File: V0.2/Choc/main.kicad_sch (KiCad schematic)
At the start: 40 parts, among them J1 USB_C_2.0, J2 JST-BAT, J3 SWD, SW1 SW_DPST_x2, SW10 SW_DPST_x2, SW11 SW_DPST_x2, SW12 SW_DPST_x2, SW13 SW_DPST_x2, SW14 SW_DPST_x2, SW15 SW_DPST_x2, SW16 SW_DPST_x2, SW17 SW_DPST_x2, SW18 SW_DPST_x2, SW19 SW_DPST_x2, SW2 SW_DPST_x2, SW20 SW_DPST_x2, SW21 SW_DPST_x2, SW3 SW_DPST_x2, SW4 SW_DPST_x2, SW5 SW_DPST_x2, SW6 SW_DPST_x2, SW7 SW_DPST_x2, SW8 SW_DPST_x2, SW9 SW_DPST_x2, U1 IP4234CZ6, U2 BQ24072, U3 MS88SF31_Min

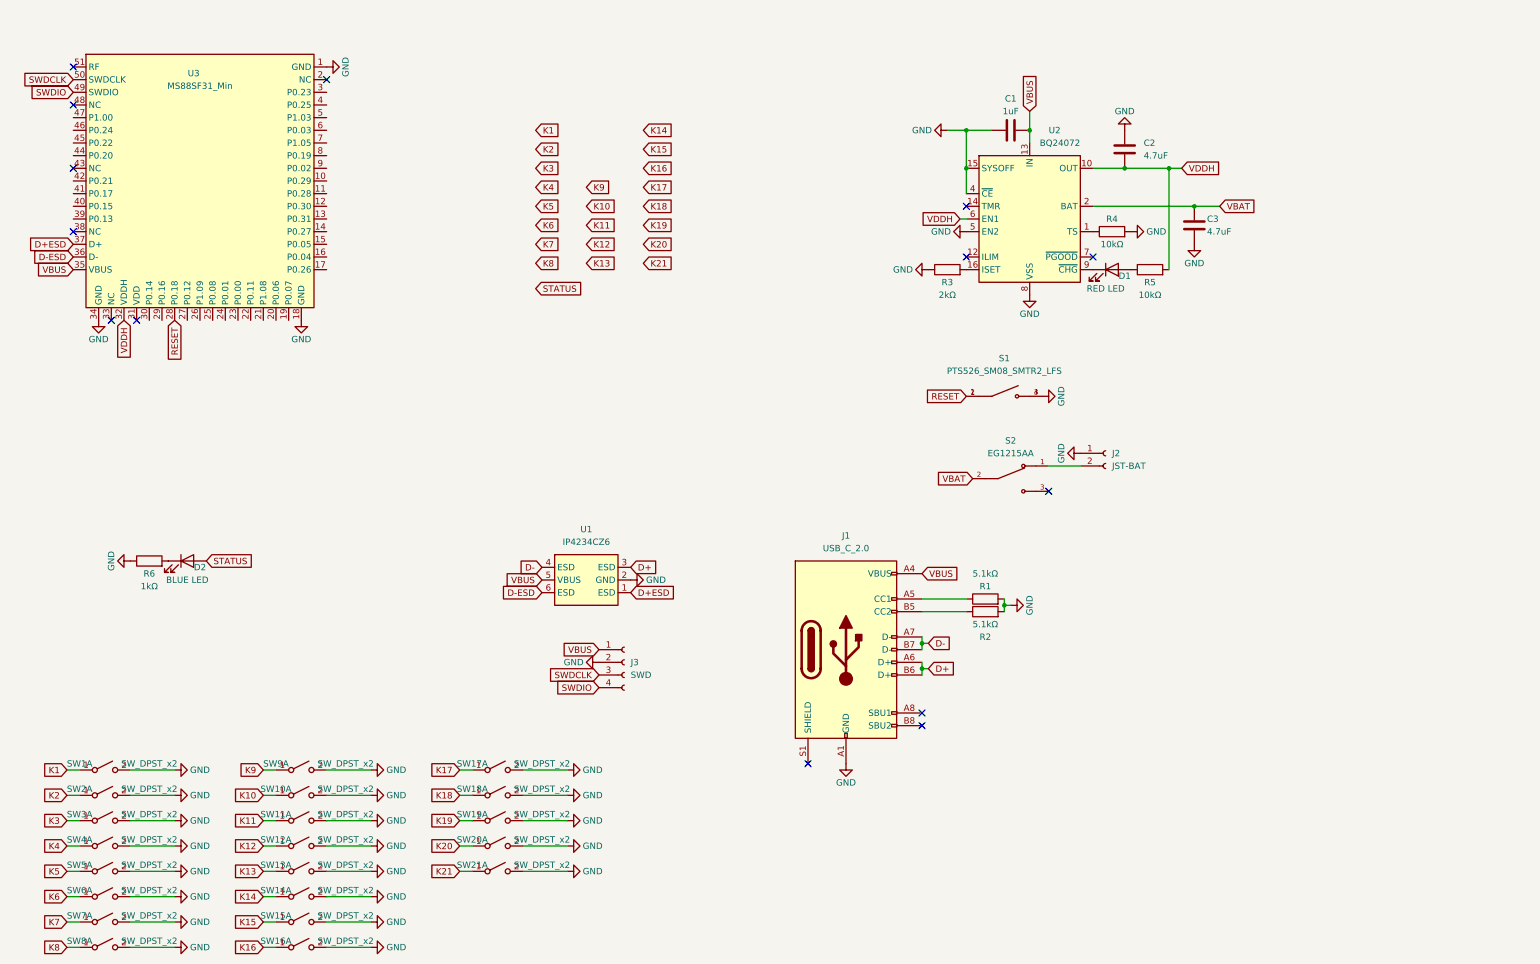
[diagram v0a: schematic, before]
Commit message: Update Readme
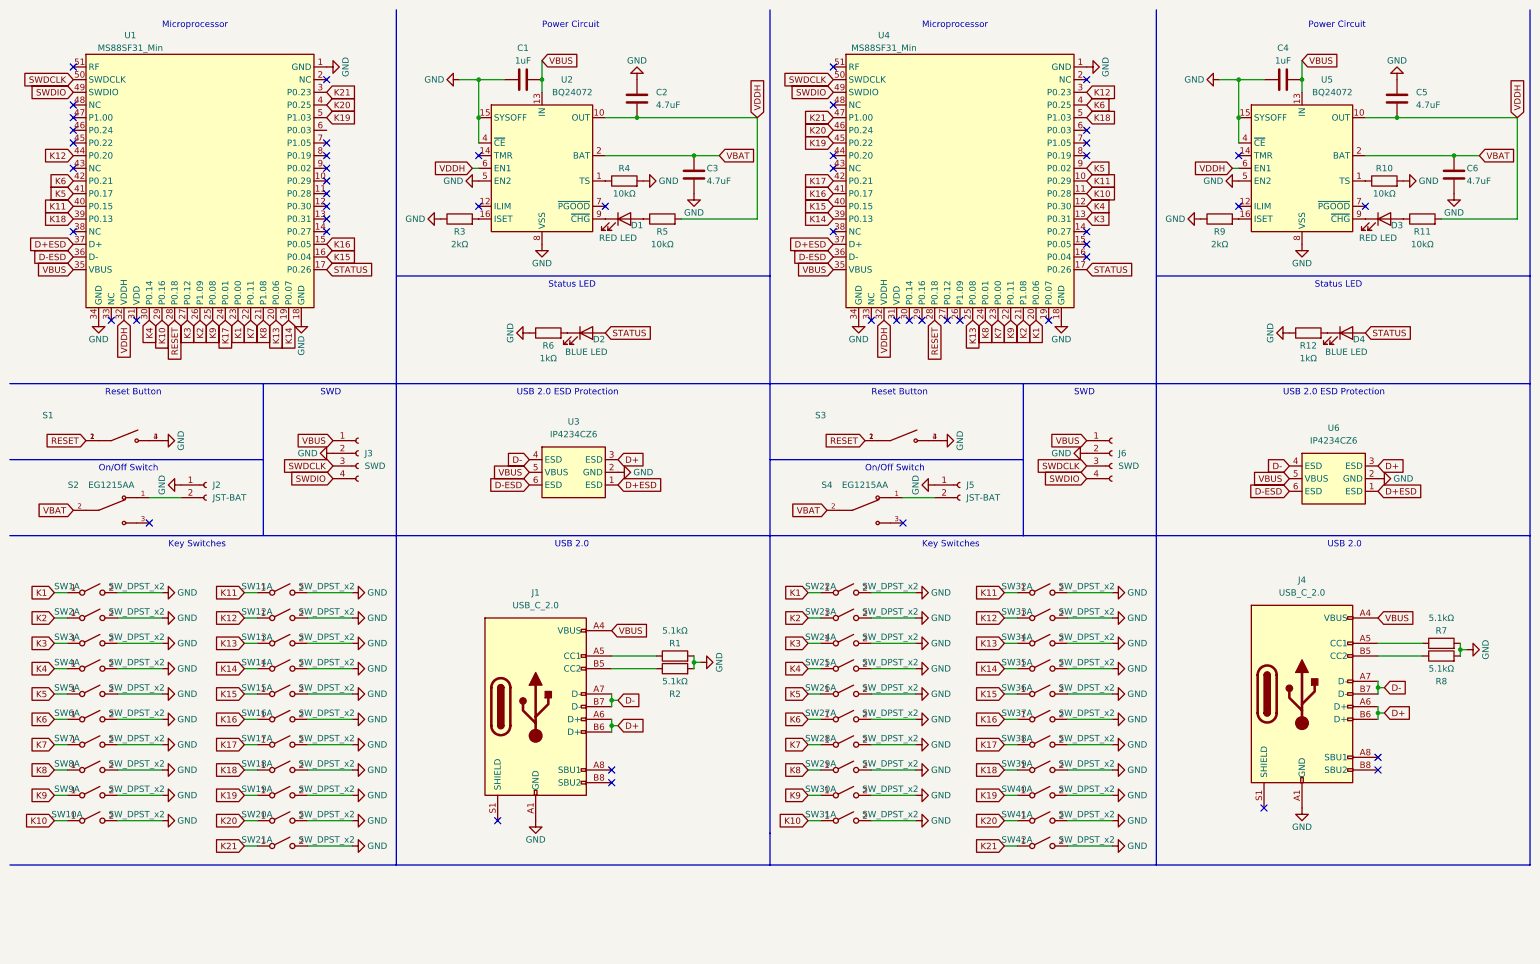
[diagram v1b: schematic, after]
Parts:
- added C4: 1uF, symbol Device:C
- added C5, C6: 4.7uF, symbol Device:C
- added D3: RED LED, symbol Device:LED
- added D4: BLUE LED, symbol Device:LED
- added J4: USB_C_2.0, symbol Connector:USB_C_Receptacle_USB2.0
- added J5: JST-BAT, symbol Connector:Conn_01x02_Female
- added J6: SWD, symbol Connector:Conn_01x04_Female
- added R10, R11: 10kΩ, symbol Device:R
- added R12: 1kΩ, symbol Device:R
- added R7, R8: 5.1kΩ, symbol Device:R
- added R9: 2kΩ, symbol Device:R
- added S3: (no value), SW_PTS526_SM08_SMTR2_LFS, symbol PTS526_SM08_SMTR2_LFS:PTS526_SM08_SMTR2_LFS
- added S4: EG1215AA, SW_EG1215AA, symbol EG1215AA:EG1215AA
- added SW22, SW23, SW24, SW25, SW26, SW27, SW28, SW29, SW30, SW31, SW32, SW33, SW34, SW35, SW36, SW37, SW38, SW39, SW40, SW41, SW42: SW_DPST_x2, symbol Switch:SW_DPST_x2
- added U4: MS88SF31_Min, symbol 0_ARognes:MS88SF31_Min
- added U5: BQ24072, Package_DFN_QFN:VQFN-16-1EP_3x3mm_P0.5mm_EP1.6x1.6mm, symbol Battery_Management:BQ24075RGT
- added U6: IP4234CZ6, symbol Nexperia:IP4234CZ6
- S1: value PTS526_SM08_SMTR2_LFS -> (none)
- renumbered U3 to U1, U1 to U3
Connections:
- net D+: now also J4.A6 (D+), J4.B6 (D+), U6.3 (ESD)
- net D+ESD: now also U4.37 (D+), U6.1 (ESD)
- net D-: now also J4.A7 (D-), J4.B7 (D-), U6.4 (ESD)
- net D-ESD: now also U4.36 (D-), U6.6 (ESD)
- net GND: now also C4.1, C5.2, C6.1, J4.A1 (GND), J4.A12 (GND), J4.B1 (GND), J4.B12 (GND), J5.1 (Pin_1), J6.2 (Pin_2), R10.2, R12.1, R7.2, R8.2, R9.1, S3.3, S3.4, SW22.2 (B), SW23.2 (B), SW24.2 (B), SW25.2 (B), SW26.2 (B), SW27.2 (B), SW28.2 (B), SW29.2 (B), SW30.2 (B), SW31.2 (B), SW32.2 (B), SW33.2 (B), SW34.2 (B), SW35.2 (B), SW36.2 (B), SW37.2 (B), SW38.2 (B), SW39.2 (B), SW40.2 (B), SW41.2 (B), SW42.2 (B), U4.1 (GND), U4.18 (GND), U4.34 (GND), U5.15 (SYSOFF), U5.17 (VSS), U5.4 (~{CE}), U5.5 (EN2), U5.8 (VSS), U6.2 (GND)
- net K1: now also U1.23 (P0.00), SW22.1 (A), U4.20 (P0.06)
- net K10: now also U1.29 (P0.16), SW31.1 (A), U4.11 (P0.28)
- net K11: now also U1.40 (P0.15), SW32.1 (A), U4.10 (P0.29)
- net K12: now also U1.44 (P0.20), SW33.1 (A), U4.3 (P0.23)
- net K13: now also U1.20 (P0.06), SW34.1 (A), U4.25 (P0.08)
- net K14: now also U1.19 (P0.07), SW35.1 (A), U4.39 (P0.13)
- net K15: now also U1.16 (P0.04), SW36.1 (A), U4.40 (P0.15)
- net K16: now also U1.15 (P0.05), SW37.1 (A), U4.41 (P0.17)
- net K17: now also U1.24 (P0.01), SW38.1 (A), U4.42 (P0.21)
- net K18: now also U1.39 (P0.13), SW39.1 (A), U4.5 (P1.03)
- net K19: now also U1.5 (P1.03), SW40.1 (A), U4.45 (P0.22)
- net K2: now also U1.26 (P1.09), SW23.1 (A), U4.21 (P1.08)
- net K20: now also U1.4 (P0.25), SW41.1 (A), U4.46 (P0.24)
- net K21: now also U1.3 (P0.23), SW42.1 (A), U4.47 (P1.00)
- net K3: now also U1.27 (P0.12), SW24.1 (A), U4.13 (P0.31)
- net K4: now also U1.30 (P0.14), SW25.1 (A), U4.12 (P0.30)
- net K5: now also U1.41 (P0.17), SW26.1 (A), U4.9 (P0.02)
- net K6: now also U1.42 (P0.21), SW27.1 (A), U4.4 (P0.25)
- net K7: now also U1.22 (P0.11), SW28.1 (A), U4.23 (P0.00)
- net K8: now also U1.21 (P1.08), SW29.1 (A), U4.24 (P0.01)
- net K9: now also U1.25 (P0.08), SW30.1 (A), U4.22 (P0.11)
- net RESET: now also S3.1, S3.2, U4.28 (P0.18)
- net STATUS: now also U1.17 (P0.26), D4.2 (A), U4.17 (P0.26)
- net SWDCLK: now also J6.3 (Pin_3), U4.50 (SWDCLK)
- net SWDIO: now also J6.4 (Pin_4), U4.49 (SWDIO)
- net VBAT: now also C6.2, S4.2, U5.2 (BAT), U5.3 (BAT)
- net VBUS: now also C4.2, J4.A4 (VBUS), J4.A9 (VBUS), J4.B4 (VBUS), J4.B9 (VBUS), J6.1 (Pin_1), U4.35 (VBUS), U5.13 (IN), U6.5 (VBUS)
- net VDDH: now also C5.1, R11.2, U4.32 (VDDH), U5.10 (OUT), U5.11 (OUT), U5.6 (EN1)
- new net: J5.2 (Pin_2), S4.1
- new net: R9.2, U5.16 (ISET)
- new net: J4.A5 (CC1), R7.1
- new net: D3.2 (A), R11.1
- new net: R10.1, U5.1 (TS)
- new net: D3.1 (K), U5.9 (~{CHG})
- new net: D4.1 (K), R12.2
- new net: J4.B5 (CC2), R8.1
- no-connect marks 14 -> 51
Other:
- note added: "Key Switches"
- note added: "Microprocessor"
- note added: "On/Off Switch"
- note added: "Power Circuit"
- note added: "Reset Button"
- note added: "SWD"
- note added: "Status LED"
- note added: "USB 2.0"
- note added: "USB 2.0 ESD Protection"
- moved on the sheet: C1, C2, C3, D1, D2, J1, J2, J3, R1, R2, R3, R4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
